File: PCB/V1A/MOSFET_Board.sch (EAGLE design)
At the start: 274 parts, among them IC301 78L05_TO-220AB-3-BR, IC302 78L05_TO-220AB-3-BR, J301 TEMP, J302 +12V, J303 CTRL, J304 FAN_MOLEX4PIN, J305 FAN_MOLEX4PIN, J306 DUT+, J307 DUT-, Q201 SIRC10DP, Q202 SIRC10DP, Q203 BC817, Q204 BC817, Q205 SIRC10DP, Q206 SIRC10DP, Q207 BC817, Q208 BC807, Q209 BC817, Q210 BC807, Q211 IXTK102N65X2, Q212 IXTK102N65X2, Q301 BC817, Q302 BC817, Q401 BC807, Q402 BC807, Q403 BC807, Q404 BC807, Q405 BC807, Q406 BC807, Q407 BC807, Q408 BC807, Q409 BC807, Q410 BC807, Q411 BC807, Q412 BC807, Q413 BC807, Q414 BC807, U201 AD420, U202 AD420, U203 LT1014I, U204 LT1014I, U205 AD620, U206 AD620, U207 AD620, U208 AD620, U209 LTC1865L, U210 LTC1865L, U301 LP2985-3.1, U302 LP2985-3.1, U303 LP2985-3.1, U304 AD620, U305 LTC1865L, U306 LTC1865L, U307 MAX743, U401 HCPL-063N, U402 HCPL-063N, U403 HCPL-063N, U404 HCPL-063N, U405 HCPL-063N, U406 HCPL-063N, U407 HCPL-063N

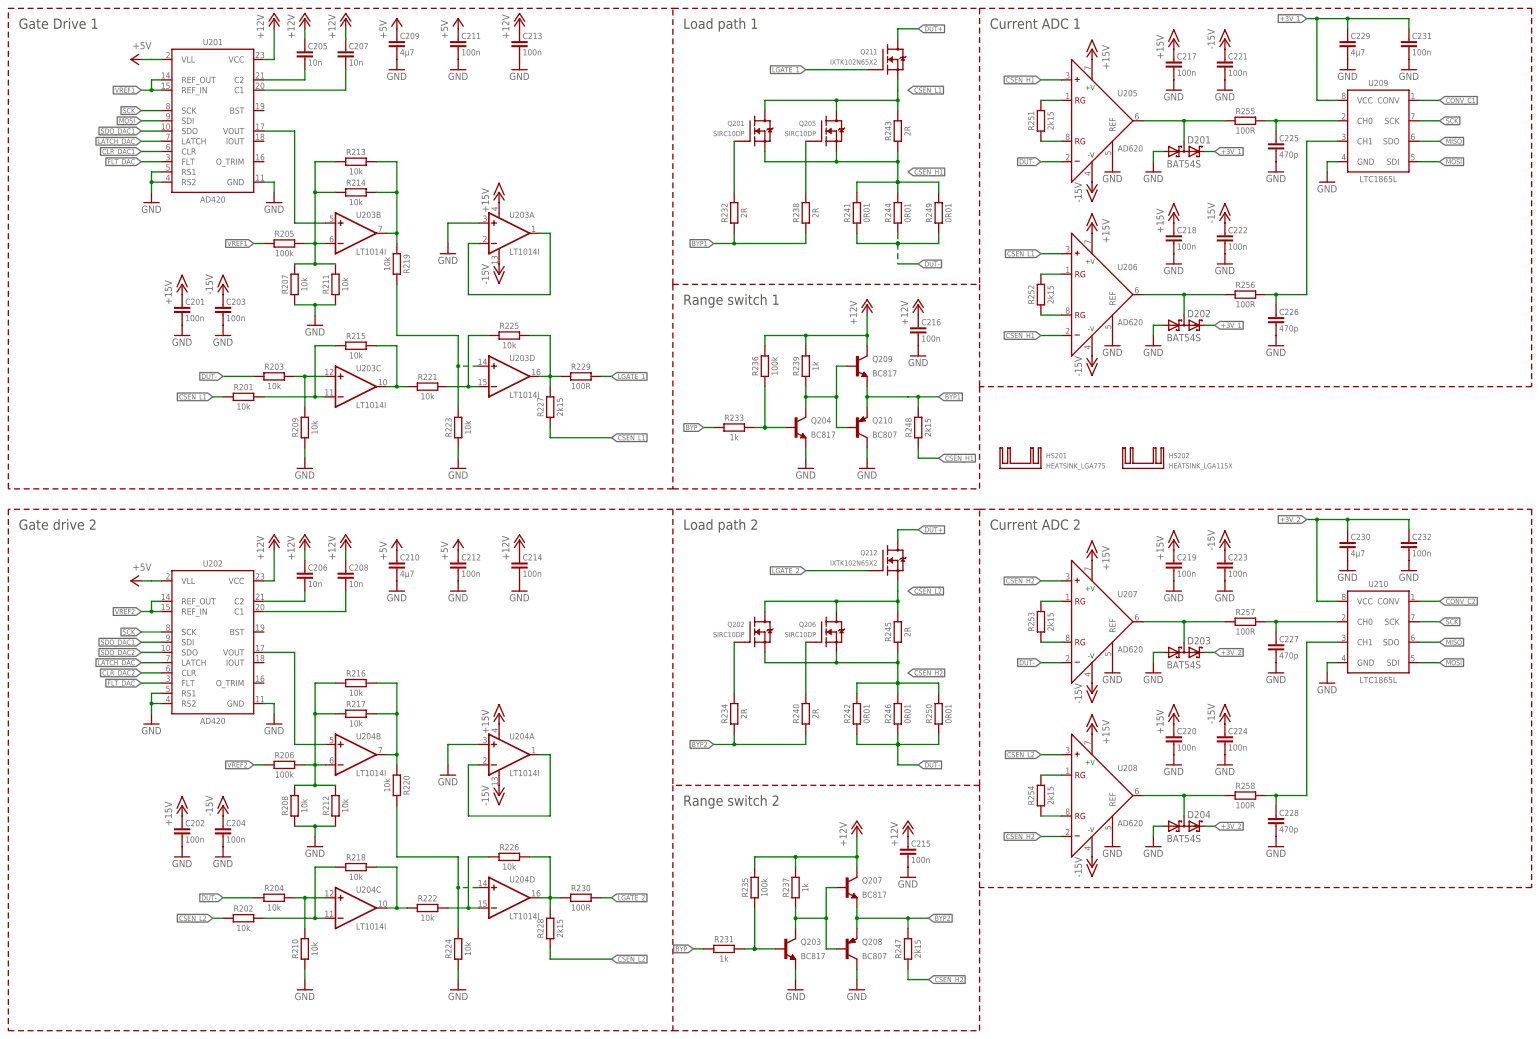
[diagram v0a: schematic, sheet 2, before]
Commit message: PCB layout
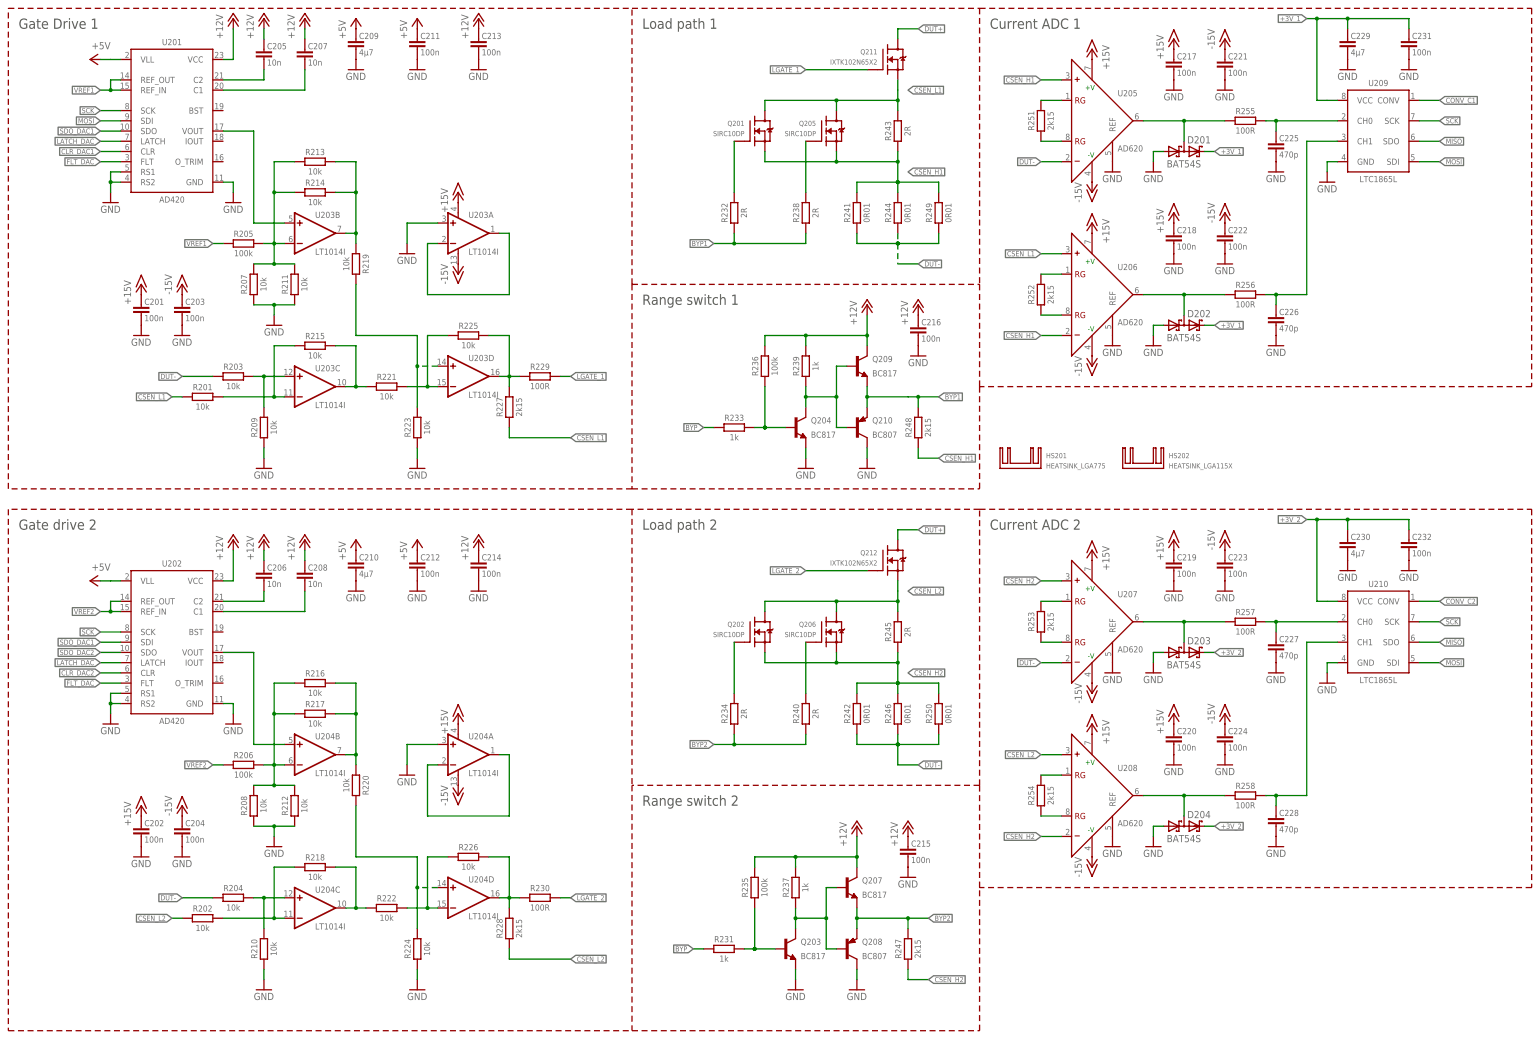
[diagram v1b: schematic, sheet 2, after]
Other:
- moved on the sheet: C201, C202, C203, C204, C205, C206, C207, C208, C209, C210, C211, C212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
